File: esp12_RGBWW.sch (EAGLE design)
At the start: 23 parts

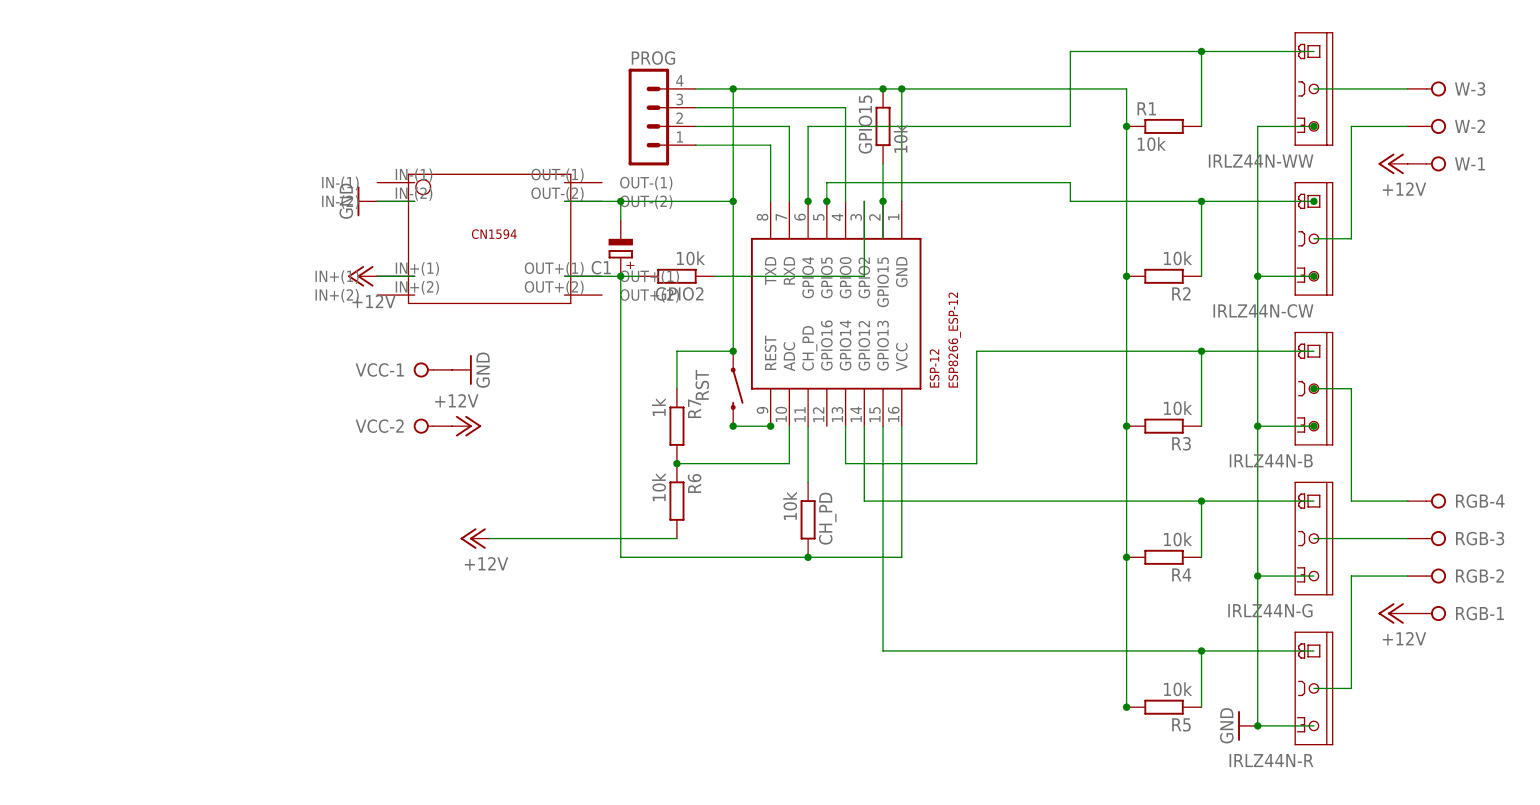
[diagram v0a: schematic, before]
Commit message: v1.2
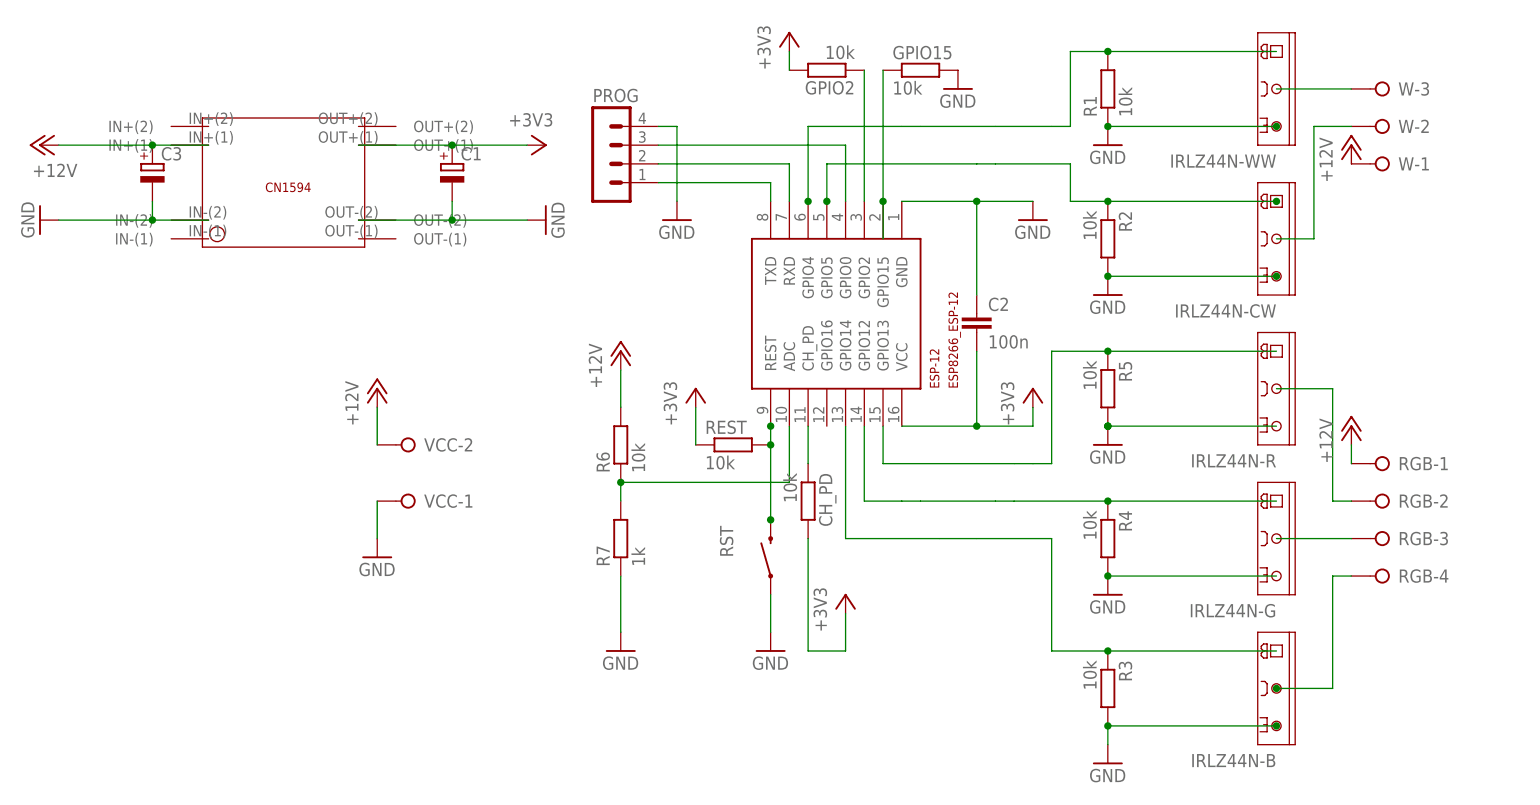
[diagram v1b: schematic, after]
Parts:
- added C2: 100n, rcl:C-EUC0805
- added C3: (no value), resistor:CPOL-EUE2.5-6
- added REST: 10k, rcl:R-EU_R0805
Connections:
- removed net GND3.3V: C1.-, DC_CONVERTER.OUT-(2), ESP-12.GND, GPIO15.2, PROG.4, R1.1, R2.2, R3.2, R4.2, R5.2, R7.1, RST.1
- removed net N$20: C1.+, CH_PD.2, DC_CONVERTER.OUT+(1), ESP-12.VCC, GPIO2.2
- new net +3V3: C1.+, C2.2, CH_PD.2, DC_CONVERTER.OUT+(1), ESP-12.VCC, GPIO2.2, REST.1
- net +12V: now also C3.+
- net GND: now also C1.-, C2.1, C3.-, DC_CONVERTER.OUT-(2), ESP-12.GND, GPIO15.2, PROG.4, R1.1, R2.2, R3.2, R4.2, R5.2, R7.1, RST.1
- net N$12: now also REST.2
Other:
- moved on the sheet: C1, CH_PD, GPIO15, GPIO2, IRLZ44N-B, IRLZ44N-CW, IRLZ44N-G, IRLZ44N-R, IRLZ44N-WW, PROG, R1, R2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
